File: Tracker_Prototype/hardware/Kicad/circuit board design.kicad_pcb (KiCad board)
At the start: 2 copper layers, 31 x 17.8 mm, 23 parts, among them J1 Conn_01x06, J2 GND, J3 3.3V, U1 MAX-M8C, U3 CMWX1ZZABZ-078, U6 MS5607-02BA

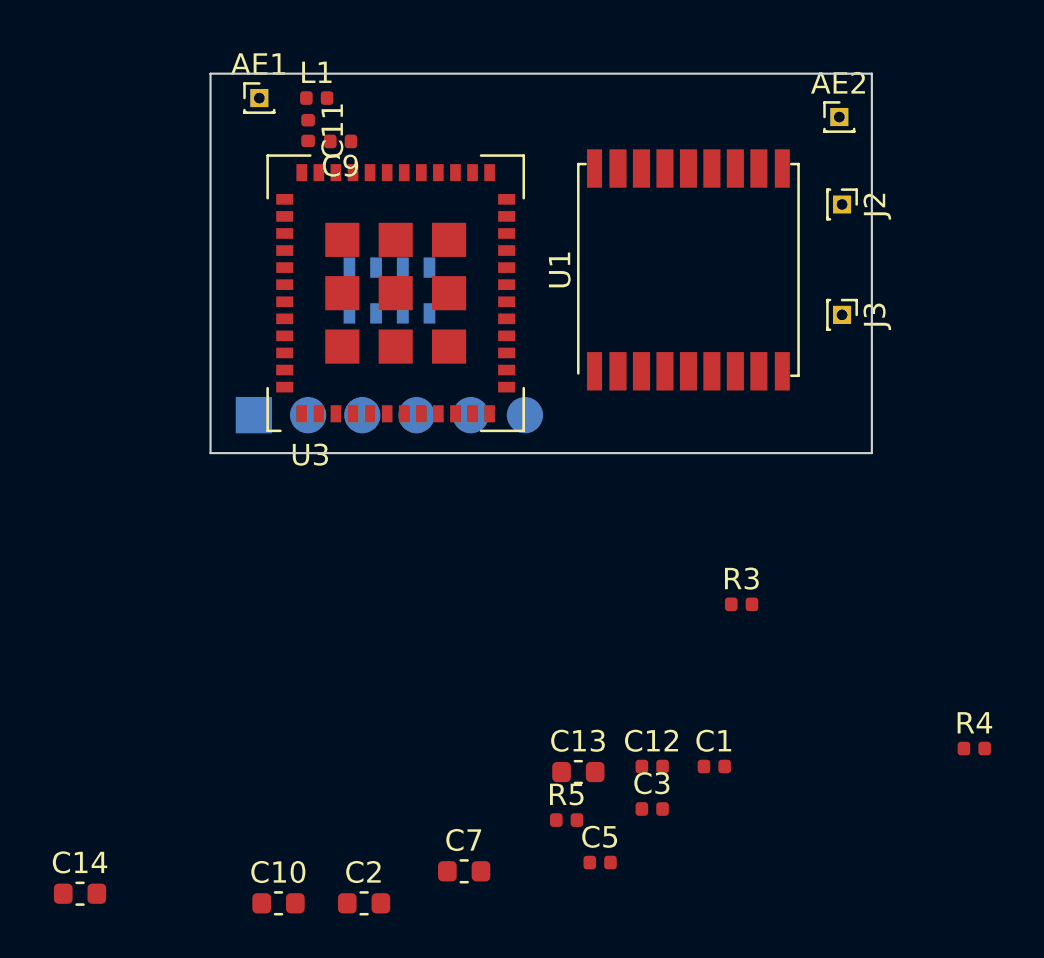
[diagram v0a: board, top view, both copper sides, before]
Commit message: Fully routed the board
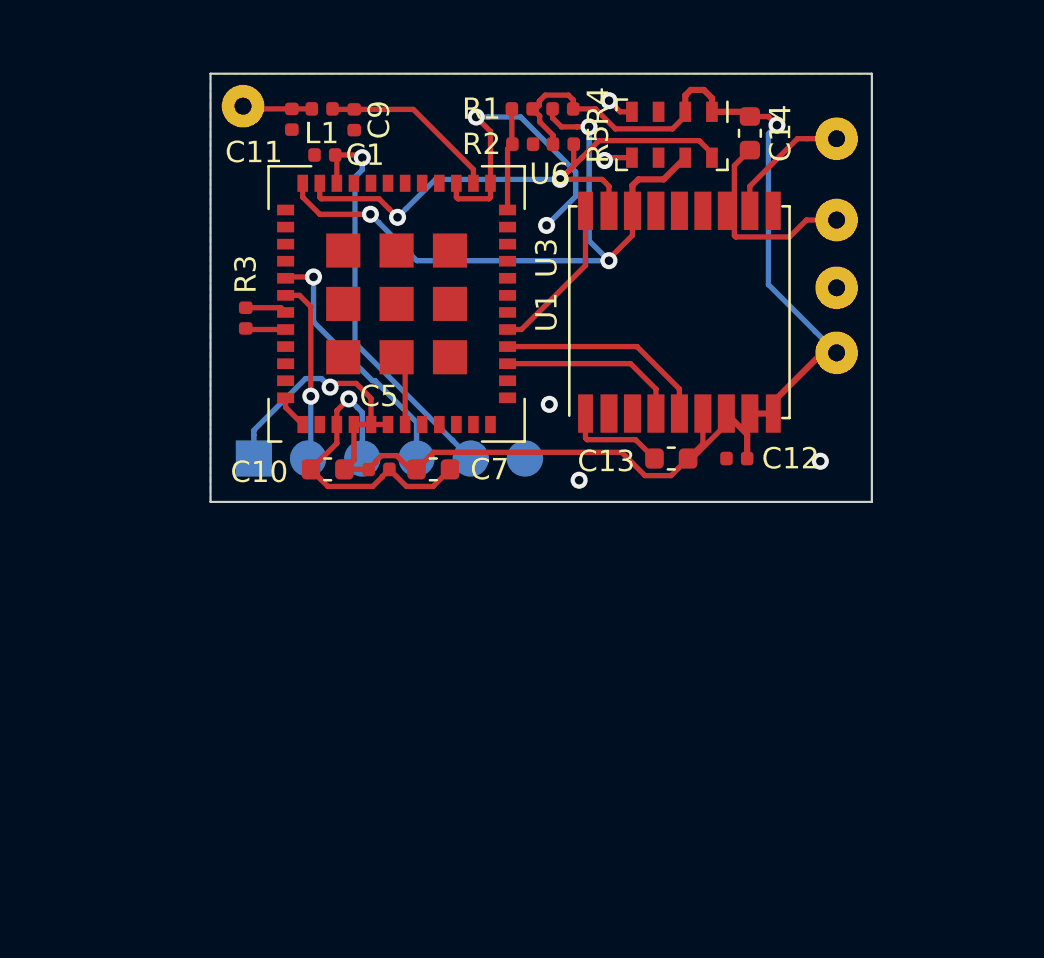
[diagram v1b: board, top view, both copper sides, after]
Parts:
- removed C2: 10uF, Capacitor_SMD:C_0603_1608Metric
- removed C3: 100nF, Capacitor_SMD:C_0402_1005Metric
- added No connection: Unconnected, Connector_Wire:SolderWirePad_1x01_Drill0.8mm, F.Cu at (296.0, 170.1)
- added R1: 100K, Resistor_SMD:R_0402_1005Metric, F.Cu at (281.3, 161.7)
- added R2: 100K, Resistor_SMD:R_0402_1005Metric, F.Cu at (281.3, 163.3)
- 3.3V: renamed from J3; footprint Connector_PinHeader_1.00mm:PinHeader_1x01_P1.00mm_Vertical -> Connector_Wire:SolderWirePad_1x01_Drill0.8mm
- AE1, AE2: footprint Connector_PinHeader_1.00mm:PinHeader_1x01_P1.00mm_Vertical -> Connector_Wire:SolderWirePad_1x01_Drill0.8mm
- GND: renamed from J2; footprint Connector_PinHeader_1.00mm:PinHeader_1x01_P1.00mm_Vertical -> Connector_Wire:SolderWirePad_1x01_Drill0.8mm
- U6: moved to F.Cu
- moved C14 47.5 mm to (292.0, 162.8), turned to 270 degrees
- moved R4 35.6 mm to (283.2, 161.7), turned to 180 degrees
- moved C1 34.0 mm to (272.1, 163.8), turned to 180 degrees
- moved R5 31.7 mm to (283.2, 163.3)
- moved R3 26.8 mm to (268.4, 171.5), turned to 270 degrees
- moved C5 21.1 mm to (274.6, 178.6)
- moved C10 20.5 mm to (272.2, 178.6), turned to 180 degrees
- moved C7 18.9 mm to (277.1, 178.6)
- moved C13 15.3 mm to (288.3, 178.1), turned to 180 degrees
- moved U6 15.1 mm to (288.3, 162.9)
- moved C12 15.0 mm to (291.4, 178.1), turned to 180 degrees
- moved J1 2.03 mm to (268.7, 178.1)
- moved U1 2.03 mm to (288.7, 171.2)
- moved 3.3V 1.80 mm to (296.0, 173.1)
- moved C9 1.20 mm to (273.4, 162.2), turned to 270 degrees
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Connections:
- J1 pad 6: (no net) -> Net-(J1-Pad6)
- U1 pad 14: (no net) -> Net-(U1-Pad14)
- U1 pad 15: (no net) -> Net-(U1-Pad15)
- U1 pad 2: (no net) -> Net-(U1-Pad2)
- U1 pad 3: (no net) -> Net-(U1-Pad3)
- U3 pad 1: (no net) -> /VDD_TCXO
- U3 pad 10: (no net) -> Net-(U3-Pad10)
- U3 pad 11: (no net) -> Net-(U3-Pad11)
- U3 pad 12: (no net) -> Net-(U3-Pad12)
- U3 pad 13: (no net) -> Net-(U3-Pad13)
- U3 pad 14: /VDD_TCXO -> Net-(U3-Pad14)
- U3 pad 18: (no net) -> Net-(U3-Pad18)
- U3 pad 19: (no net) -> Net-(U3-Pad19)
- U3 pad 2: (no net) -> Net-(U3-Pad2)
- U3 pad 20: (no net) -> Net-(U3-Pad20)
- U3 pad 21: (no net) -> Net-(U3-Pad21)
- U3 pad 22: (no net) -> Net-(U3-Pad22)
- U3 pad 23: (no net) -> Net-(U3-Pad23)
- U3 pad 24: (no net) -> /V_SOLAR
- U3 pad 28: (no net) -> Net-(U3-Pad28)
- U3 pad 29: (no net) -> Net-(U3-Pad29)
- U3 pad 30: (no net) -> Net-(U3-Pad30)
- U3 pad 31: (no net) -> Net-(U3-Pad31)
- U3 pad 32: (no net) -> Net-(U3-Pad32)
- U3 pad 33: (no net) -> Net-(U3-Pad33)
- U3 pad 37: (no net) -> Net-(U3-Pad37)
- U3 pad 38: (no net) -> Net-(U3-Pad38)
- U3 pad 39: (no net) -> Net-(U3-Pad39)
- U3 pad 40: (no net) -> Net-(U3-Pad40)
- U3 pad 45: (no net) -> Net-(U3-Pad45)
- U3 pad 46: (no net) -> Net-(U3-Pad46)
- U3 pad 47: (no net) -> Net-(U3-Pad47)
- U3 pad 8: (no net) -> Net-(U3-Pad8)
- U3 pad 9: (no net) -> Net-(U3-Pad9)
- U6 pad 6: (no net) -> Net-(U6-Pad6)
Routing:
- net +3V3: track 0.00 -> 76.2 mm, vias 0 -> 2
- net GND: track 0.00 -> 52.5 mm, vias 0 -> 8
- net /I2C1_SDA: track 0.00 -> 32.2 mm, vias 0 -> 3
- net /I2C1_SCL: track 0.00 -> 26.8 mm, vias 0 -> 2
- net /RESET: track 0.00 -> 19.2 mm, vias 0 -> 1
- net /SWDIO: track 0.00 -> 11.9 mm, vias 0 -> 1
- net /GPS_EXTINT: track 0.00 -> 10.0 mm
- net /GPS_TIMEPULSE: track 0.00 -> 8.59 mm
- net /SWCLK: track 0.00 -> 8.57 mm, vias 0 -> 1
- net Net-(C9-Pad1): track 0.00 -> 8.43 mm
- net /GPS_SAFEBOOT: track 0.00 -> 7.46 mm
- net Net-(AE2-Pad1): track 0.00 -> 6.14 mm
- net /V_SOLAR: track 0.00 -> 4.84 mm
- net Net-(AE1-Pad1): track 0.00 -> 3.27 mm
- net Net-(R3-Pad1): track 0.00 -> 1.96 mm
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- added copper zone on B.Cu, net GND
- added copper zone on F.Cu, net GND
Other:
- board size 31 x 17.8 mm -> 31 x 20.1 mm
- net class FETs removed
- net class Power: trace_width 2 -> 0.5
- net class sense removed
